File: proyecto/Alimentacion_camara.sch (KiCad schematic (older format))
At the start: 4 parts

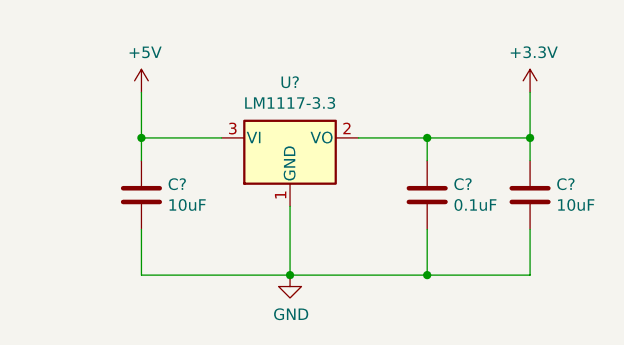
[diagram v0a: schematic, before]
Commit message: Add files via upload
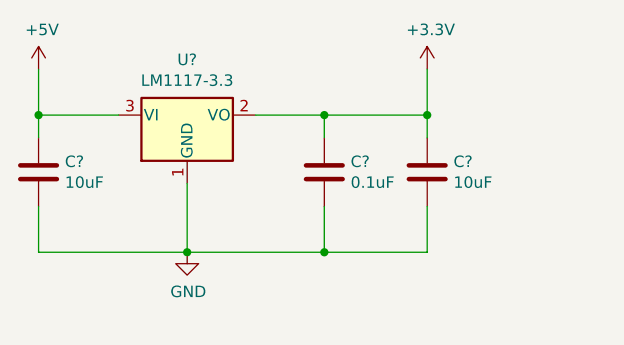
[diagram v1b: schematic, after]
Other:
- moved on the sheet: C?, U?
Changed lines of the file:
@@
 $Descr A4 11693 8268
 encoding utf-8
-Sheet 5 7
+Sheet 7 7
 Title ""
 Date ""
@@
 L Regulator_Linear:LM1117-3.3 U?
 U 1 1 5E9D90F6
-P 4700 3450
+P 4250 3350
 AR Path="/5E9D90F6" Ref="U?"  Part="1"
 AR Path="/5E9BC166/5E9D90F6" Ref="U?"  Part="1"
 AR Path="/5EA3D59C/5E9D90F6" Ref="U?"  Part="1"
-F 0 "U?" H 4700 3692 50  0000 C CNN
-F 1 "LM1117-3.3" H 4700 3601 50  0000 C CNN
-F 2 "" H 4700 3450 50  0001 C CNN
-F 3 "http://www.ti.com/lit/ds/symlink/lm1117.pdf" H 4700 3450 50  0001 C CNN
-	1    4700 3450
+F 0 "U?" H 4250 3592 50  0000 C CNN
+F 1 "LM1117-3.3" H 4250 3501 50  0000 C CNN
+F 2 "" H 4250 3350 50  0001 C CNN
+F 3 "http://www.ti.com/lit/ds/symlink/lm1117.pdf" H 4250 3350 50  0001 C CNN
+	1    4250 3350
 	1    0    0    -1
 $EndComp
@@
 L Device:C C?
 U 1 1 5E9D90FC
-P 4050 3700
+P 3600 3600
 AR Path="/5E9D90FC" Ref="C?"  Part="1"
 AR Path="/5E9BC166/5E9D90FC" Ref="C?"  Part="1"
 AR Path="/5EA3D59C/5E9D90FC" Ref="C?"  Part="1"
-F 0 "C?" H 4165 3746 50  0000 L CNN
-F 1 "10uF" H 4165 3655 50  0000 L CNN
-F 2 "" H 4088 3550 50  0001 C CNN
-F 3 "~" H 4050 3700 50  0001 C CNN
-	1    4050 3700
+F 0 "C?" H 3715 3646 50  0000 L CNN
+F 1 "10uF" H 3715 3555 50  0000 L CNN
+F 2 "" H 3638 3450 50  0001 C CNN
+F 3 "~" H 3600 3600 50  0001 C CNN
+	1    3600 3600
 	1    0    0    -1
 $EndComp
@@
 L Device:C C?
 U 1 1 5E9D9102
-P 5300 3700
+P 4850 3600
 AR Path="/5E9D9102" Ref="C?"  Part="1"
 AR Path="/5E9BC166/5E9D9102" Ref="C?"  Part="1"
 AR Path="/5EA3D59C/5E9D9102" Ref="C?"  Part="1"
-F 0 "C?" H 5415 3746 50  0000 L CNN
-F 1 "0.1uF" H 5415 3655 50  0000 L CNN
-F 2 "" H 5338 3550 50  0001 C CNN
-F 3 "~" H 5300 3700 50  0001 C CNN
-	1    5300 3700
+F 0 "C?" H 4965 3646 50  0000 L CNN
+F 1 "0.1uF" H 4965 3555 50  0000 L CNN
+F 2 "" H 4888 3450 50  0001 C CNN
+F 3 "~" H 4850 3600 50  0001 C CNN
+	1    4850 3600
 	1    0    0    -1
 $EndComp
@@
 L Device:C C?
 U 1 1 5E9D9108
-P 5750 3700
+P 5300 3600
 AR Path="/5E9D9108" Ref="C?"  Part="1"
 AR Path="/5E9BC166/5E9D9108" Ref="C?"  Part="1"
 AR Path="/5EA3D59C/5E9D9108" Ref="C?"  Part="1"
-F 0 "C?" H 5865 3746 50  0000 L CNN
-F 1 "10uF" H 5865 3655 50  0000 L CNN
-F 2 "" H 5788 3550 50  0001 C CNN
-F 3 "~" H 5750 3700 50  0001 C CNN
-	1    5750 3700
+F 0 "C?" H 5415 3646 50  0000 L CNN
+F 1 "10uF" H 5415 3555 50  0000 L CNN
+F 2 "" H 5338 3450 50  0001 C CNN
+F 3 "~" H 5300 3600 50  0001 C CNN
+	1    5300 3600
 	1    0    0    -1
 $EndComp
 Wire Wire Line
-	4400 3450 4050 3450
+	3950 3350 3600 3350
 Wire Wire Line
-	4050 3550 4050 3450
+	3600 3450 3600 3350
 Wire Wire Line
-	5300 3550 5300 3450
-Connection ~ 5300 3450
+	4850 3450 4850 3350
+Connection ~ 4850 3350
 Wire Wire Line
-	5300 3450 5000 3450
+	4850 3350 4550 3350
 Wire Wire Line
-	5750 3550 5750 3450
+	5300 3450 5300 3350
 Wire Wire Line
-	5750 3450 5300 3450
+	5300 3350 4850 3350
 $Comp
 L power:GND #PWR?
 U 1 1 5E9D911B
-P 4700 4050
+P 4250 3950
 AR Path="/5E9D911B" Ref="#PWR?"  Part="1"
 AR Path="/5E9BC166/5E9D911B" Ref="#PWR?"  Part="1"
 AR Path="/5EA3D59C/5E9D911B" Ref="#PWR?"  Part="1"
-F 0 "#PWR?" H 4700 3800 50  0001 C CNN
-F 1 "GND" H 4705 3877 50  0000 C CNN
-F 2 "" H 4700 4050 50  0001 C CNN
-F 3 "" H 4700 4050 50  0001 C CNN
-	1    4700 4050
+F 0 "#PWR?" H 4250 3700 50  0001 C CNN
+F 1 "GND" H 4255 3777 50  0000 C CNN
+F 2 "" H 4250 3950 50  0001 C CNN
+F 3 "" H 4250 3950 50  0001 C CNN
+	1    4250 3950
 	1    0    0    -1
 $EndComp
 Wire Wire Line
-	5750 4050 5300 4050
-Connection ~ 4700 4050
+	5300 3950 4850 3950
+Connection ~ 4250 3950
 Wire Wire Line
-	4700 3750 4700 4050
+	4250 3650 4250 3950
 Wire Wire Line
-	5300 3850 5300 4050
-Connection ~ 5300 4050
+	4850 3750 4850 3950
+Connection ~ 4850 3950
 Wire Wire Line
-	5300 4050 4700 4050
+	4850 3950 4250 3950
 Wire Wire Line
-	4050 3850 4050 4050
+	3600 3750 3600 3950
 Wire Wire Line
-	4050 4050 4700 4050
+	3600 3950 4250 3950
 Wire Wire Line
-	5750 3850 5750 4050
+	5300 3750 5300 3950
 $Comp
 L power:+3.3V #PWR?
 U 1 1 5E9C6FA9
-P 5750 3250
+P 5300 3150
 AR Path="/5E9BC166/5E9C6FA9" Ref="#PWR?"  Part="1"
 AR Path="/5EA3D59C/5E9C6FA9" Ref="#PWR?"  Part="1"
-F 0 "#PWR?" H 5750 3100 50  0001 C CNN
-F 1 "+3.3V" H 5765 3423 50  0000 C CNN
-F 2 "" H 5750 3250 50  0001 C CNN
-F 3 "" H 5750 3250 50  0001 C CNN
-	1    5750 3250
+F 0 "#PWR?" H 5300 3000 50  0001 C CNN
+F 1 "+3.3V" H 5315 3323 50  0000 C CNN
+F 2 "" H 5300 3150 50  0001 C CNN
+F 3 "" H 5300 3150 50  0001 C CNN
+	1    5300 3150
 	1    0    0    -1
 $EndComp
@@
 L power:+5V #PWR?
 U 1 1 5E9C79B9
-P 4050 3250
+P 3600 3150
 AR Path="/5E9BC166/5E9C79B9" Ref="#PWR?"  Part="1"
 AR Path="/5EA3D59C/5E9C79B9" Ref="#PWR?"  Part="1"
-F 0 "#PWR?" H 4050 3100 50  0001 C CNN
-F 1 "+5V" H 4065 3423 50  0000 C CNN
-F 2 "" H 4050 3250 50  0001 C CNN
-F 3 "" H 4050 3250 50  0001 C CNN
-	1    4050 3250
+F 0 "#PWR?" H 3600 3000 50  0001 C CNN
+F 1 "+5V" H 3615 3323 50  0000 C CNN
+F 2 "" H 3600 3150 50  0001 C CNN
+F 3 "" H 3600 3150 50  0001 C CNN
+	1    3600 3150
 	1    0    0    -1
 $EndComp
 Wire Wire Line
-	5750 3250 5750 3450
-Connection ~ 5750 3450
+	5300 3150 5300 3350
+Connection ~ 5300 3350
 Wire Wire Line
-	4050 3450 4050 3250
-Connection ~ 4050 3450
+	3600 3350 3600 3150
+Connection ~ 3600 3350
 $EndSCHEMATC
